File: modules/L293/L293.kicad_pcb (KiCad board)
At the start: 2 copper layers, 40.6 x 40.6 mm, 40 parts, among them J1 2, J10 11, J11 12, J12 13, J13 A0, J14 A1, J15 A2, J16 A3, J17 A4, J18 A5, J19 Vcc, J2 3, J20 Gnd, J21 Pwr, J22 M1, J23 M2, J3 4, J4 5, J5 6, J6 7, J7 8, J8 9, J9 10, U1 74LVC1G79, U2 74LVC1G79, U3 74LVC1G79, U4 74LVC1G79, U5 L293D, U6 L4940

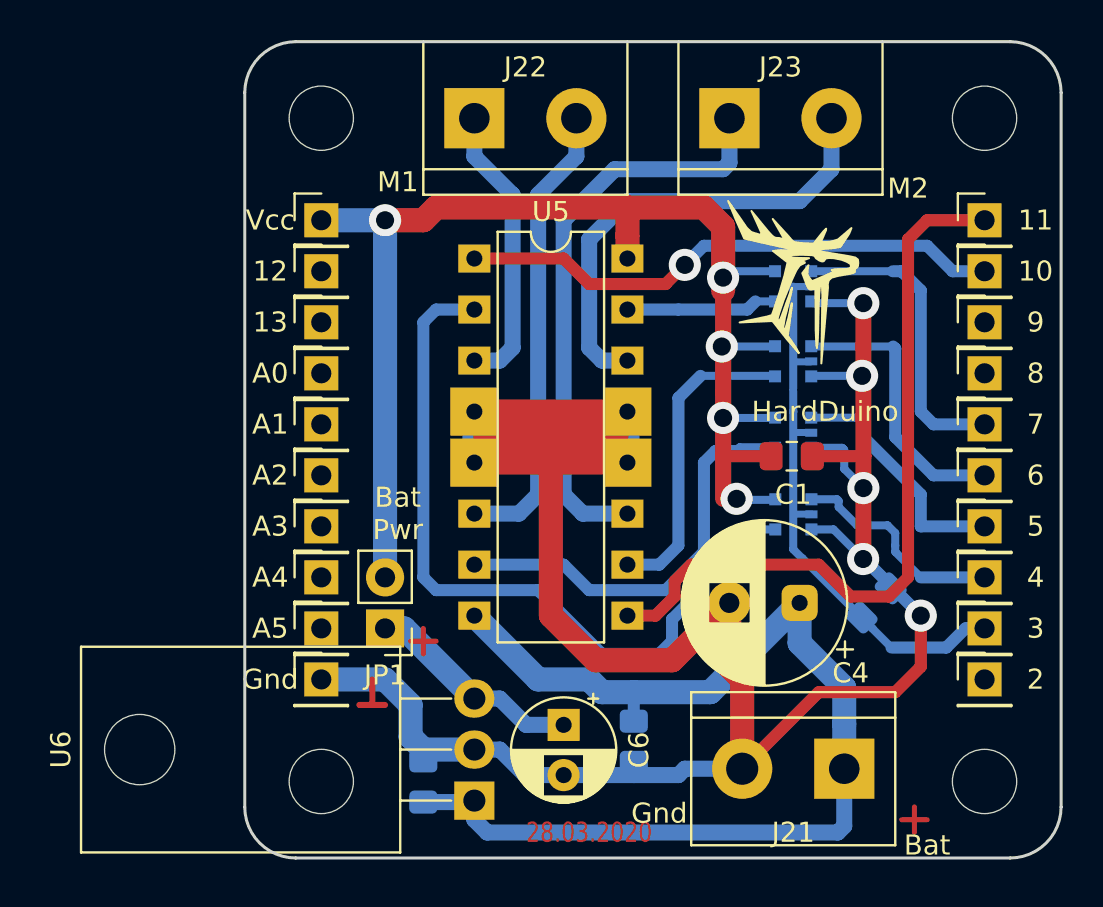
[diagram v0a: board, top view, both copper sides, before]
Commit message: L293 in work.
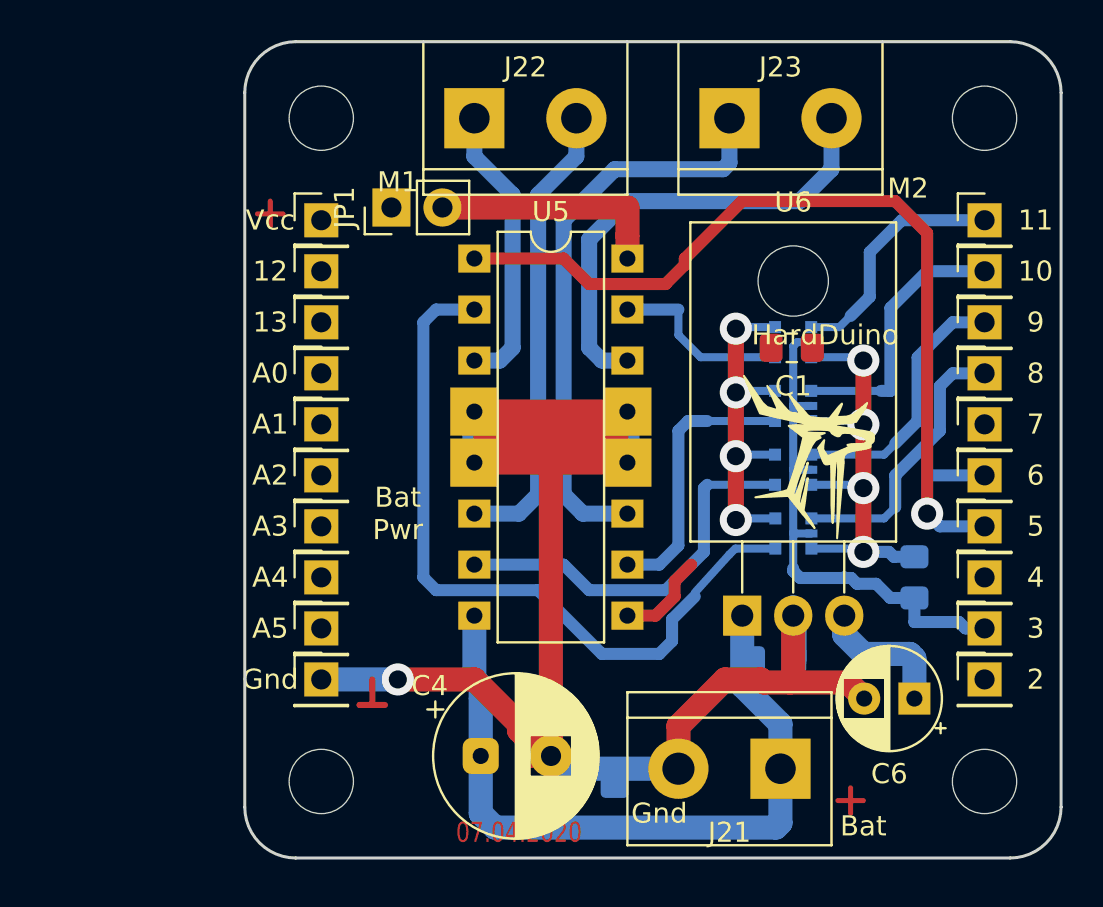
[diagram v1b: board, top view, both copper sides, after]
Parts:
- moved JP1 21.0 mm to (96.2, 36.2), turned to 90 degrees
- moved C5 18.5 mm to (115.3, 58.7), turned to 0 degrees
- moved C4 17.6 mm to (100.6, 63.5), turned to 0 degrees
- moved C6 17.5 mm to (122.2, 60.6), turned to 180 degrees
- moved U6 16.2 mm to (113.7, 56.5), turned to 0 degrees
- moved C1 5.40 mm to (116.1, 43.2)
- moved C2 3.38 mm to (107.3, 66.0), turned to 270 degrees
- moved J21 3.18 mm to (115.6, 64.1)
- moved U4 2.78 mm to (119.0, 41.3)
- moved R1 2.29 mm to (122.2, 54.6), turned to 270 degrees
- moved U3 2.22 mm to (119.0, 44.5)
- moved U2 1.84 mm to (119.0, 47.6)
- moved U1 0.95 mm to (119.1, 50.8)
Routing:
- net /PWM1: track 0.00 -> 42.7 mm, vias 0 -> 1
- net Net-(J10-Pad1): track 37.6 -> 0.00 mm
- net VCC: track 66.6 -> 29.2 mm, vias 5 -> 4
- net Net-(J9-Pad1): track 27.2 -> 0.00 mm, vias 1 -> 0
- net GND: track 117.0 -> 97.9 mm
- net Net-(C2-Pad2): track 55.4 -> 37.0 mm
- net Net-(J6-Pad1): track 15.3 -> 0.00 mm
- net Net-(J5-Pad1): track 13.9 -> 0.00 mm
- net /M1+: track 0.00 -> 13.8 mm
- net /M2+: track 0.00 -> 13.5 mm
- net /M1-: track 0.00 -> 13.2 mm
- net Net-(J4-Pad1): track 12.2 -> 0.00 mm
- net /M2-: track 0.00 -> 12.1 mm
- net Net-(J3-Pad1): track 11.0 -> 0.00 mm
- net /PWM2: track 0.00 -> 7.22 mm
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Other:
- board text added: "07.04.2020"
- board text removed: "28.03.2020"
